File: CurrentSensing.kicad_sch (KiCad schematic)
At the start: 9 parts, among them SW1 SW_SPDT, SW2 SW_SPDT, SW3 SW_SPDT

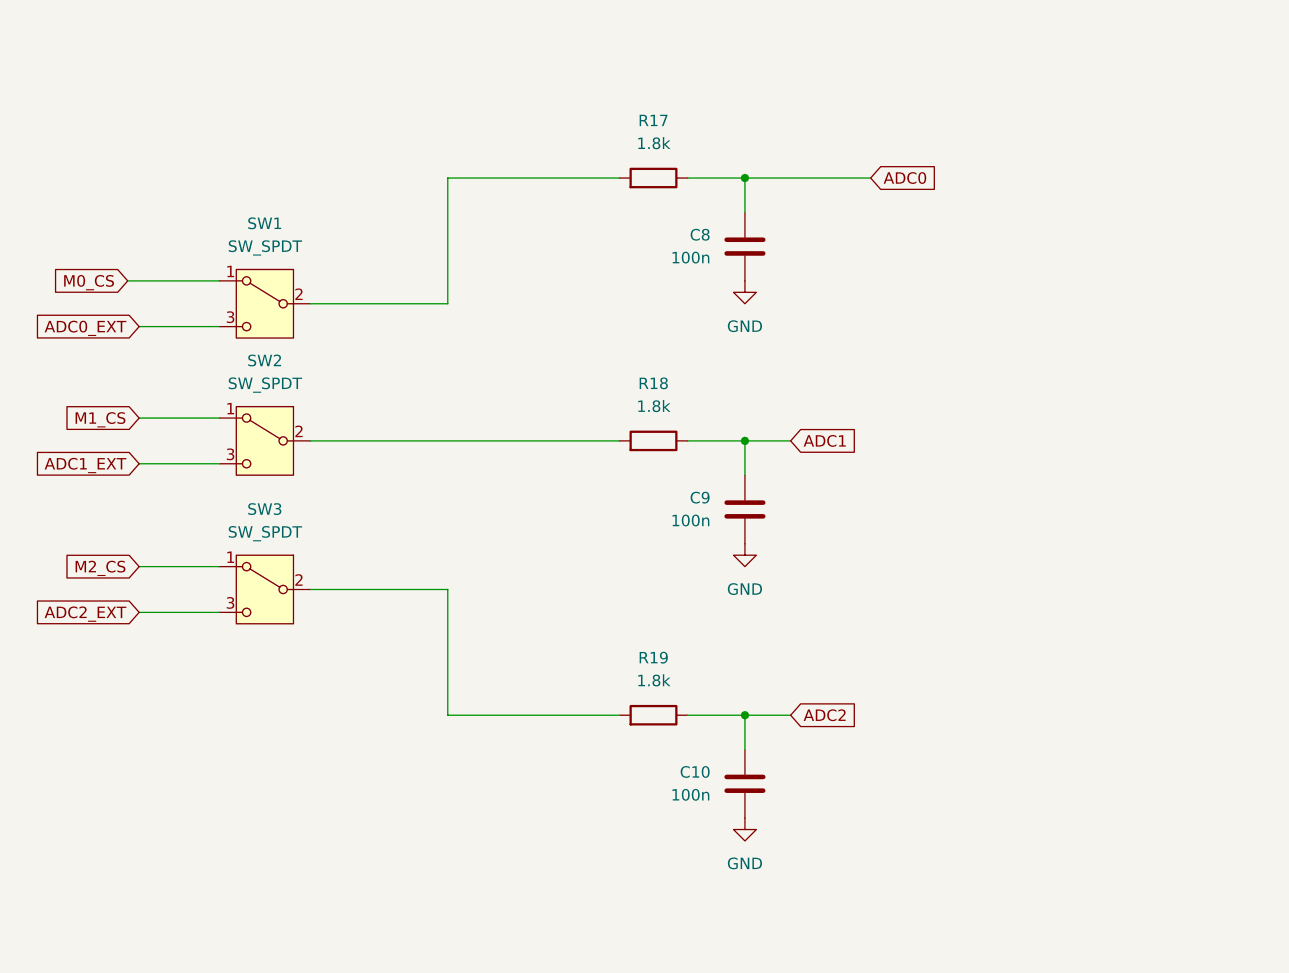
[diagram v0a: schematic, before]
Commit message: Add files via upload
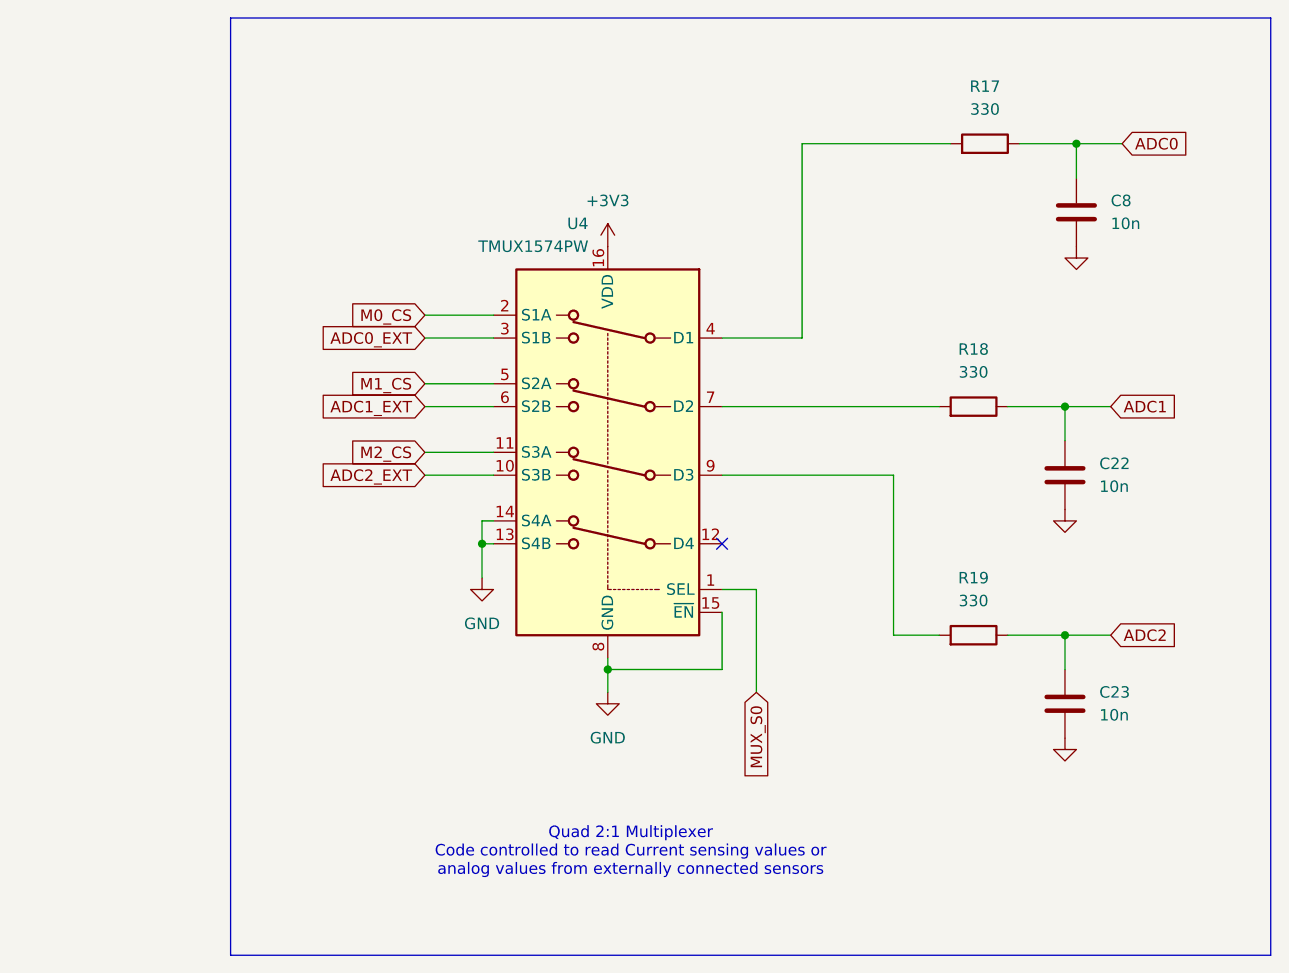
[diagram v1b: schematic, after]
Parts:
- removed C10, C9: 100n, Capacitor_SMD:C_0603_1608Metric_Pad1.08x0.95mm_HandSolder, symbol Device:C
- removed SW1, SW2, SW3: SW_SPDT, Button_Switch_SMD:SW_SPST_Panasonic_EVQPL_3PL_5PL_PT_A15, symbol Switch:SW_SPDT
- added C22, C23: 10n, Capacitor_SMD:C_0603_1608Metric_Pad1.08x0.95mm_HandSolder, symbol Device:C
- added U4: TMUX1574PW, Package_SO:TSSOP-16_4.4x5mm_P0.65mm, symbol Analog_Switch:TMUX1574PW
- C8: value 100n -> 10n
- R17, R18, R19: value 1.8k -> 330
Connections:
- net ADC0_EXT: now also U4.3 (S1B)
- net ADC1: now also C22.1
- net ADC1_EXT: now also U4.6 (S2B)
- net ADC2: now also C23.1
- net ADC2_EXT: now also U4.10 (S3B)
- net GND: now also C22.2, C23.2, U4.13 (S4B), U4.14 (S4A), U4.15 (~{EN}), U4.8 (GND)
- net M0_CS: now also U4.2 (S1A)
- net M1_CS: now also U4.5 (S2A)
- net M2_CS: now also U4.11 (S3A)
- net at R18.2: now also U4.7 (D2)
- net at R19.2: now also U4.9 (D3)
- net at R17.2: now also U4.4 (D1)
- new net +3V3: U4.16 (VDD)
- new net MUX_S0: U4.1 (SEL)
- no-connect marks 0 -> 1
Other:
- note added: "Quad 2:1 Multiplexer Code controlled to read Current sensing values or analog values from externally connected sensors"
- moved on the sheet: C8, R17
